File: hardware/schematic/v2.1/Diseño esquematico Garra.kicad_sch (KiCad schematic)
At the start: 20 parts

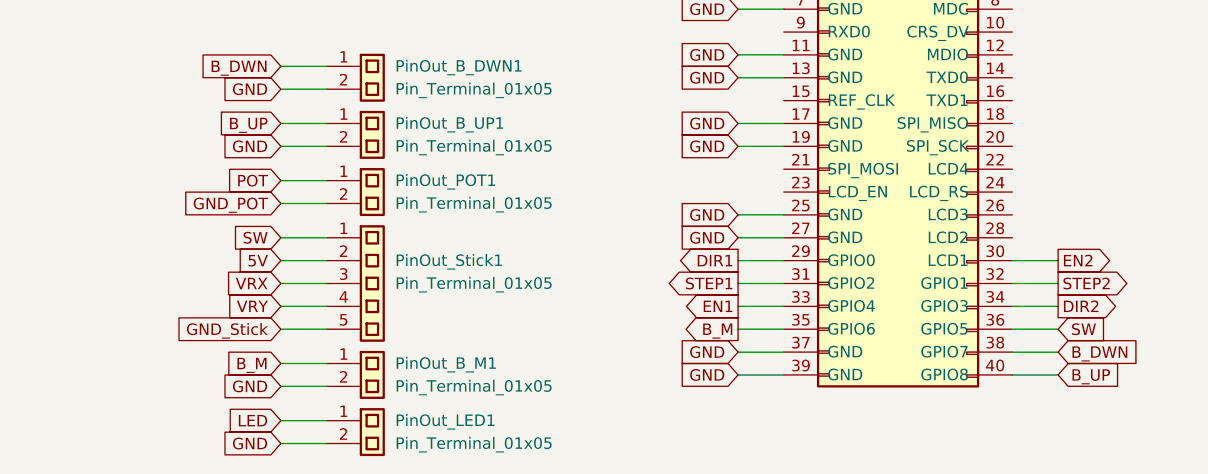
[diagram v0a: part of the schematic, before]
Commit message: fix: PDF
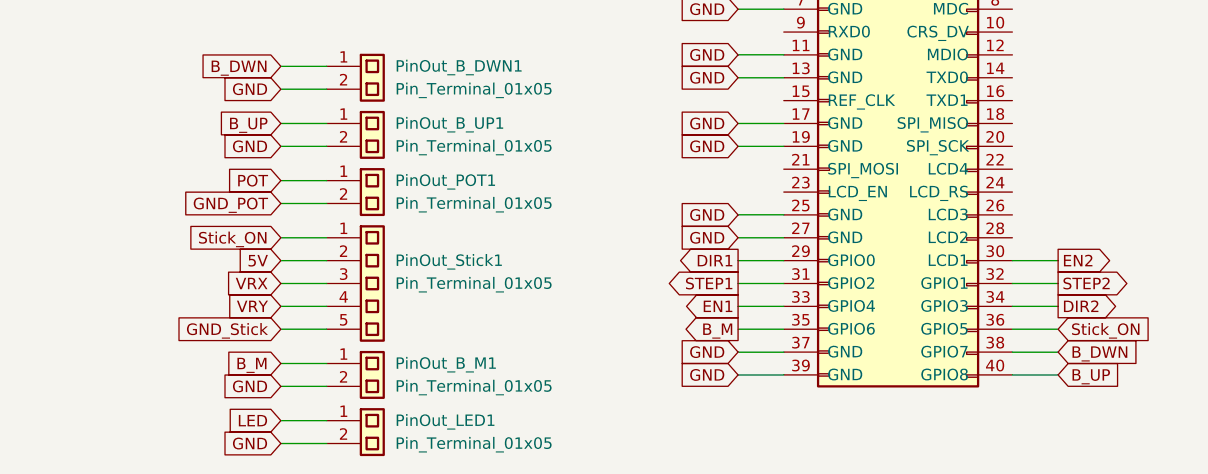
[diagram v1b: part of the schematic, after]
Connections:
- net SW renamed Stick_ON
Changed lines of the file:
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@@
 		)
 	)
-	(global_label "SW"
+	(global_label "Stick_ON"
 		(shape input)
 		(at 182.88 133.35 180)
@@
 		)
 	)
-	(global_label "SW"
+	(global_label "Stick_ON"
 		(shape input)
 		(at 269.24 143.51 0)
